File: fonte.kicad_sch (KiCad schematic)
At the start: 13 parts

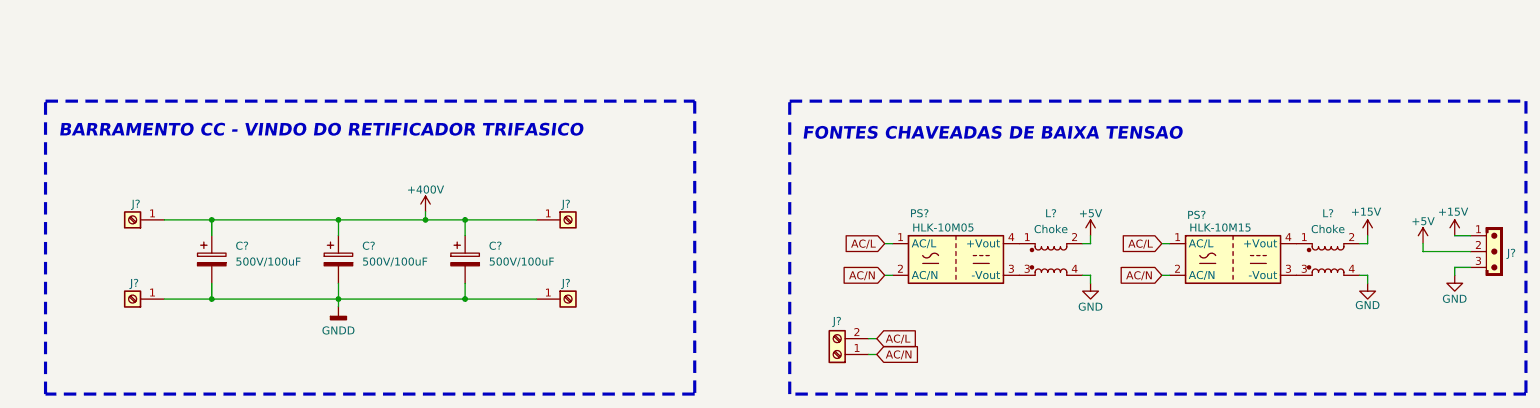
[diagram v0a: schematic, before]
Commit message: midsave
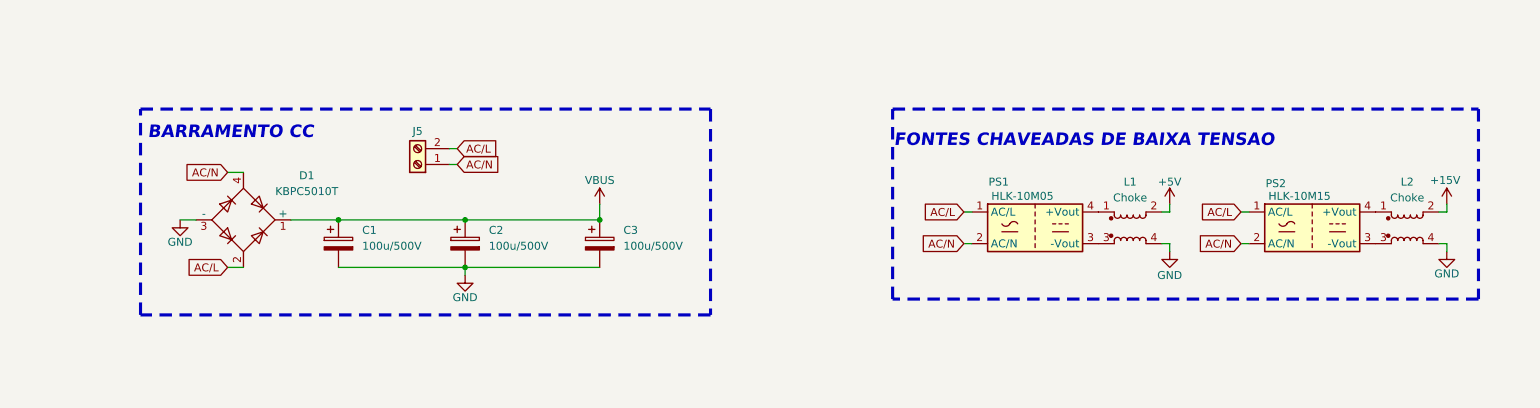
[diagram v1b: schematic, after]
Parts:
- removed C? (x3): 500V/100uF, symbol Device:C_Polarized
- removed J? (x4): Screw_Terminal_01x01, symbol Connector:Screw_Terminal_01x01
- removed J?: JST_03, Connector_JST:JST_EH_B3B-EH-A_1x03_P2.50mm_Vertical, symbol PCM_SL_Connectors:JST_03
- added C1, C2, C3: 100u/500V, Capacitor_THT:CP_Radial_D22.0mm_P10.00mm_SnapIn, symbol Device:C_Polarized
- added D1: KBPC5010T, Diode_THT:Diode_Bridge_DIGITRON_KBPC_T, symbol Diode_Bridge:KBPC5010T
- J5: renamed from J?; footprint (none) -> TerminalBlock_Phoenix:TerminalBlock_Phoenix_MKDS-1,5-2_1x02_P5.00mm_Horizontal
- L1, L2: renamed from L?; footprint (none) -> Inductor_THT:L_CommonMode_Toroid_Vertical_L19.3mm_W10.8mm_Px6.35mm_Py15.24mm_Bourns_8100
- gave numbers to parts that had none: 2
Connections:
- net AC/L: now also D1.2
- net AC/N: now also D1.4
- net GND: now also C1.2, C2.2, C3.2, D1.3 (-)
- new net VBUS: C1.1, C2.1, C3.1, D1.1 (+)
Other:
- note added: "BARRAMENTO CC"
- note removed: "BARRAMENTO CC - VINDO DO RETIFICADOR TRIFASICO"
- moved on the sheet: J5, L1, L2, PS1, PS2

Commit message: f
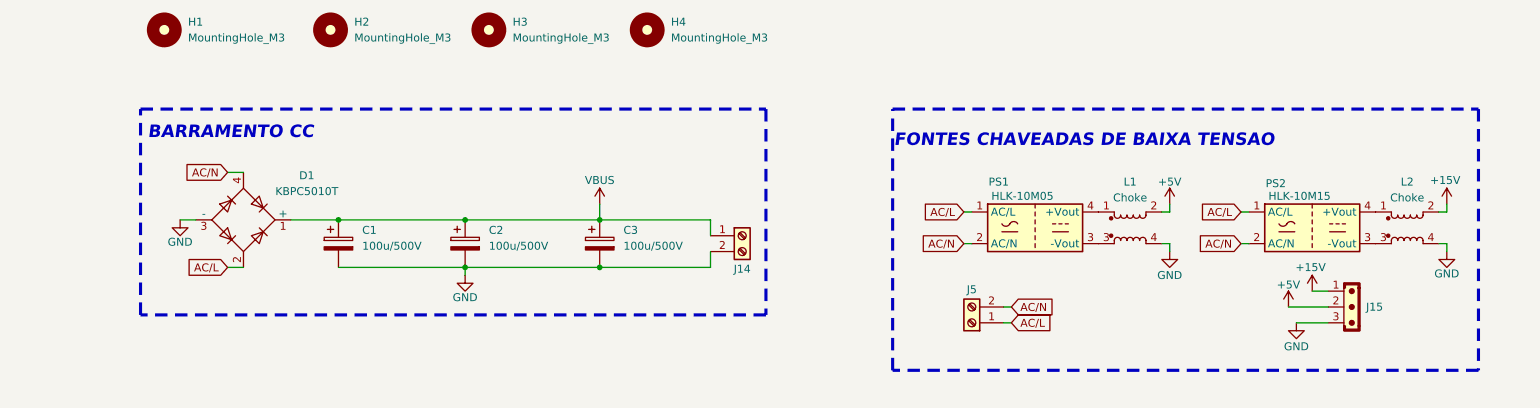
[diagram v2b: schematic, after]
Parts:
- added H1, H2, H3, H4: MountingHole_M3, MountingHole:MountingHole_3.2mm_M3, symbol PCM_SL_Mechanical:MountingHole_M3
- added J14: Screw_Terminal_01x02, TerminalBlock_Phoenix:TerminalBlock_Phoenix_MKDS-1,5-2_1x02_P5.00mm_Horizontal, symbol Connector:Screw_Terminal_01x02
- added J15: JST_03, Connector_JST:JST_EH_B3B-EH-A_1x03_P2.50mm_Vertical, symbol PCM_SL_Connectors:JST_03
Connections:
- net +15V: now also J15.1
- net +5V: now also J15.2
- net AC/L: now also J5.1 (Pin_1); no longer J5.2 (Pin_2)
- net AC/N: now also J5.2 (Pin_2); no longer J5.1 (Pin_1)
- net GND: now also J14.2 (Pin_2), J15.3
- net VBUS: now also J14.1 (Pin_1)
